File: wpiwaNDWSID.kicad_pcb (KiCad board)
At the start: 2 copper layers, 85.8 x 30 mm, 28 parts, among them J1 USB_C_Receptacle_USB2.0_16P, J2 Conn_01x02, J3 Conn_01x04, J4 Conn_01x06, SW1 SW_Push, SW2 SW_Push, U1 AP63205WU, U2 AP7363-33D-13, U3 ESP32-S3-WROOM-1, U4 74AHCT125

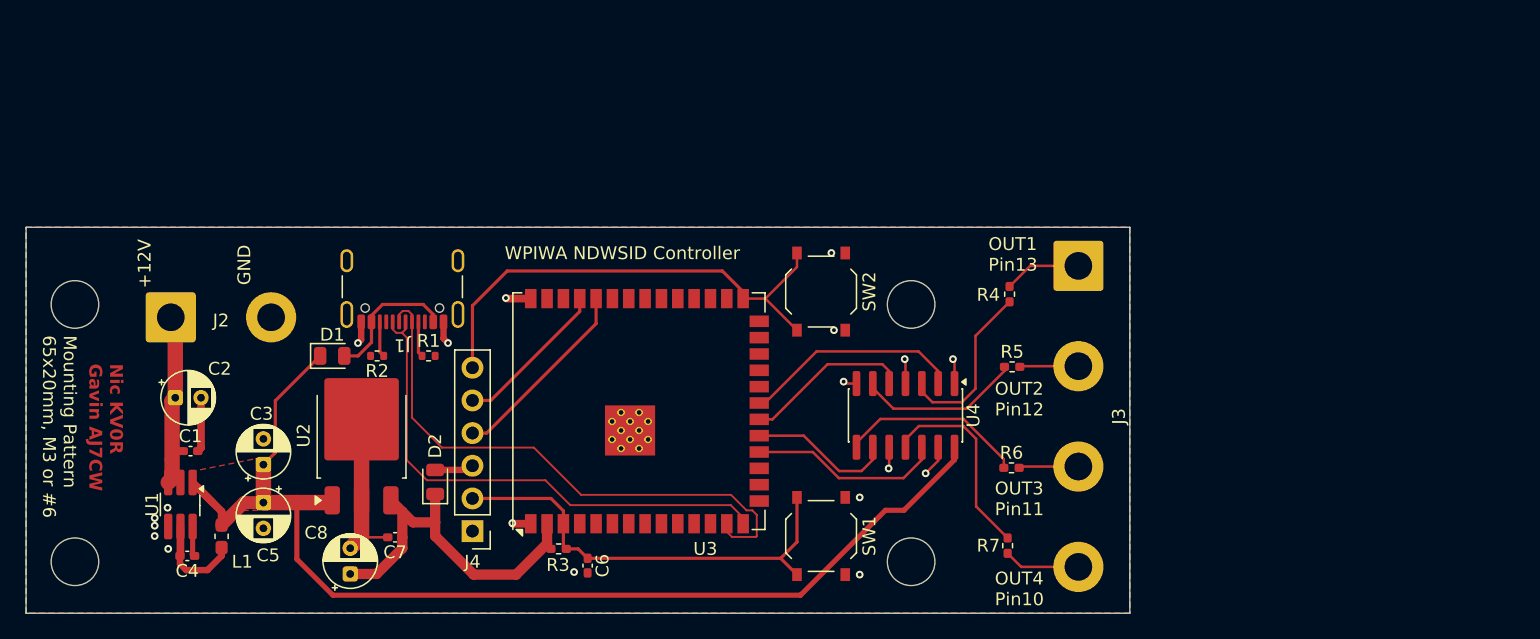
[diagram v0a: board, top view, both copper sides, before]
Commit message: rev 2
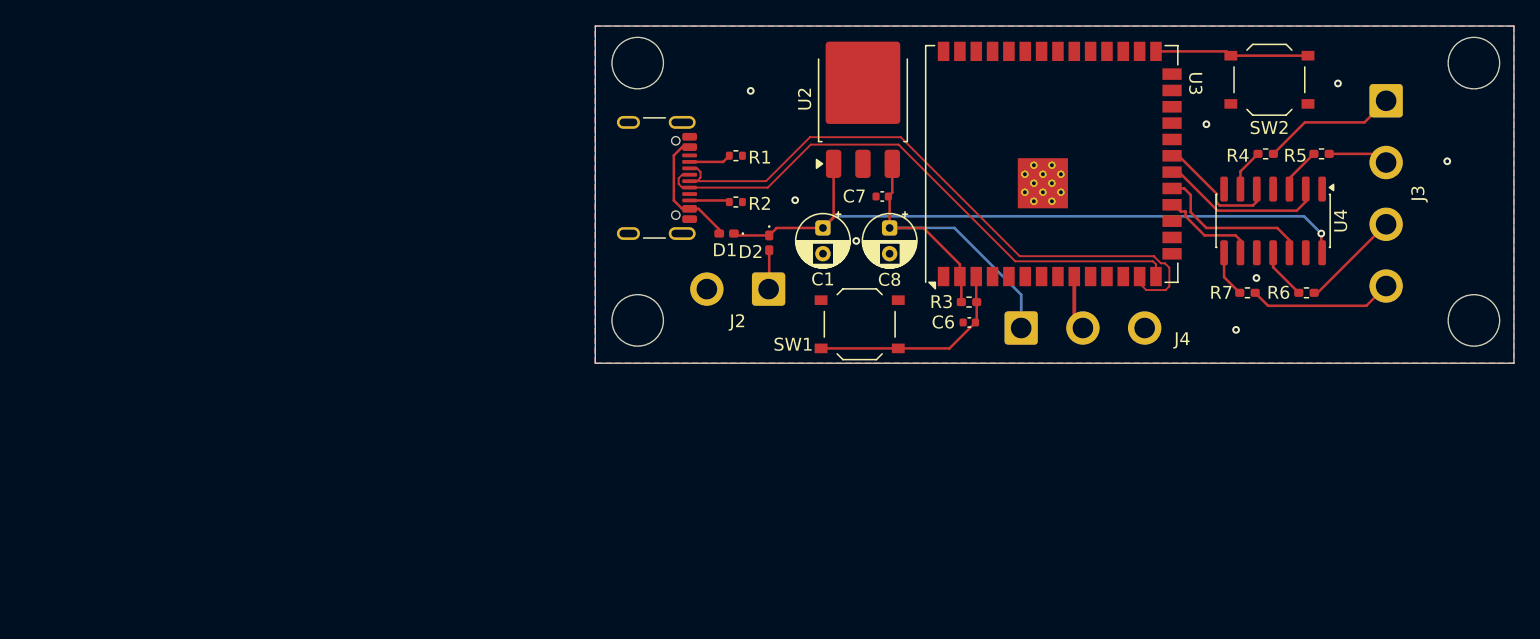
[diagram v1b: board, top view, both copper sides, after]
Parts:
- removed C2: 10uF, Capacitor_THT:CP_Radial_D4.0mm_P2.00mm
- removed C3, C5: 22uF, Capacitor_THT:CP_Radial_D4.0mm_P2.00mm
- removed C4: 0.1uF, Capacitor_SMD:C_0402_1005Metric_Pad0.74x0.62mm_HandSolder
- removed L1: 4.7uH, Inductor_SMD:L_0603_1608Metric_Pad1.05x0.95mm_HandSolder
- removed U1: AP63205WU, Package_TO_SOT_SMD:TSOT-23-6_HandSoldering
- C1: value 0.1uF -> 22uF; footprint Capacitor_SMD:C_0402_1005Metric_Pad0.74x0.62mm_HandSolder -> Capacitor_THT:CP_Radial_D4.0mm_P2.00mm
- C6, C7: footprint Capacitor_SMD:C_0402_1005Metric_Pad0.74x0.62mm_HandSolder -> Capacitor_SMD:C_0402_1005Metric
- D1, D2: footprint Diode_SMD:D_0805_2012Metric -> Diode_SMD:D_0402_1005Metric_Pad0.77x0.64mm_HandSolder
- J2: footprint Connector_Wire:SolderWire-1.5sqmm_1x02_P7.8mm_D1.7mm_OD3.9mm -> Connector_Wire:SolderWire-0.75sqmm_1x02_P4.8mm_D1.25mm_OD2.3mm
- J3: footprint Connector_Wire:SolderWire-1.5sqmm_1x04_P7.8mm_D1.7mm_OD3.9mm -> Connector_Wire:SolderWire-0.75sqmm_1x04_P4.8mm_D1.25mm_OD2.3mm
- J4: value Conn_01x06 -> Conn_01x03; footprint Connector_PinHeader_2.54mm:PinHeader_1x06_P2.54mm_Vertical -> Connector_Wire:SolderWire-0.75sqmm_1x03_P4.8mm_D1.25mm_OD2.3mm
- moved C1 52.1 mm to (180.1, 97.1), turned to -90 degrees
- moved C8 49.8 mm to (185.3, 97.1), turned to -90 degrees
- moved U2 46.9 mm to (183.3, 87.0)
- moved J2 46.5 mm to (175.9, 101.8), turned to 180 degrees
- moved C7 46.2 mm to (184.8, 94.6)
- moved J4 45.5 mm to (195.6, 104.8), turned to 0 degrees
- moved SW2 38.5 mm to (214.8, 85.5), turned to 180 degrees
- moved U3 37.4 mm to (197.9, 92.1)
- moved R3 37.2 mm to (191.5, 102.8)
- moved C6 35.2 mm to (191.5, 104.4), turned to 180 degrees
- moved U4 32.3 mm to (215.1, 96.5)
- moved D1 32.1 mm to (172.7, 97.5), turned to 180 degrees
- moved D2 31.9 mm to (176.0, 98.2), turned to -90 degrees
- moved R2 30.3 mm to (173.4, 95.0), turned to 0 degrees
- moved R5 29.2 mm to (218.9, 91.3)
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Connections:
- C1 pad 1: +12V -> +5V
- C6 pad 1: Net-(J4-Pin_2) -> Net-(U3-EN)
- D2 pad 1: +3.3V -> +5V
- J2 pad 1: +12V -> Net-(D2-A)
- J4 pad 1: GND -> +3.3V
- J4 pad 2: Net-(J4-Pin_2) -> /ESP32/RELAY
- J4 pad 3: Net-(D2-A) -> GND
- R3 pad 2: Net-(J4-Pin_2) -> Net-(U3-EN)
- SW1 pad 2: Net-(J4-Pin_2) -> Net-(U3-EN)
- SW2 pad 2: Net-(J4-Pin_6) -> Net-(U3-IO0)
- U3 pad 26: unconnected-(U3-IO45-Pad26) -> GND
- U3 pad 27: Net-(J4-Pin_6) -> Net-(U3-IO0)
- U3 pad 3: Net-(J4-Pin_2) -> Net-(U3-EN)
- U3 pad 36: Net-(J4-Pin_4) -> unconnected-(U3-RXD0-Pad36)
- U3 pad 37: Net-(J4-Pin_5) -> unconnected-(U3-TXD0-Pad37)
- U3 pad 9: unconnected-(U3-IO16-Pad9) -> /ESP32/RELAY
- U4 pad 11: Net-(R7-Pad1) -> Net-(R6-Pad1)
- U4 pad 12: /ESP32/LED_4 -> /ESP32/LED_3
- U4 pad 2: /ESP32/LED_1 -> /ESP32/LED_2
- U4 pad 3: Net-(R4-Pad1) -> Net-(R5-Pad1)
- U4 pad 5: /ESP32/LED_2 -> /ESP32/LED_1
- U4 pad 6: Net-(R5-Pad1) -> Net-(R4-Pad1)
- U4 pad 8: Net-(R6-Pad1) -> Net-(R7-Pad1)
- U4 pad 9: /ESP32/LED_3 -> /ESP32/LED_4
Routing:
- net Net-(J4-Pin_6): track 37.9 -> 0.00 mm
- net +5V: track 90.6 -> 53.7 mm, vias 0 -> 1
- net Net-(J4-Pin_2): track 35.0 -> 0.00 mm
- net GND: track 34.2 -> 0.00 mm, vias 19 -> 8
- net Net-(U3-EN): track 0.00 -> 16.5 mm
- net Net-(J4-Pin_4): track 15.1 -> 0.00 mm
- net +12V: track 14.6 -> 0.00 mm
- net Net-(J4-Pin_5): track 12.2 -> 0.00 mm
- net Net-(R7-Pad1): track 15.7 -> 3.62 mm
- net Net-(U3-IO0): track 0.00 -> 12.0 mm
- net Net-(R6-Pad1): track 14.5 -> 3.94 mm
- net Net-(R4-Pad1): track 13.4 -> 3.30 mm
- net Net-(R5-Pad1): track 12.8 -> 3.52 mm
- net /ESP32/LED_1: track 17.2 -> 9.68 mm
- net Net-(U1-SW): track 7.46 -> 0.00 mm
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- removed copper zone on F.Cu, net +5V
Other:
- board size 85.8 x 30 mm -> 71.4 x 26.2 mm
- board text removed: "+12V"
- board text removed: "GND"
- board text removed: "Mounting Pattern 65x20mm, M3 or #6"
- board text removed: "Nic KV0R Gavin AJ7CW"
- board text removed: "OUT1 Pin13"
- board text removed: "OUT2 Pin12"
- board text removed: "OUT3 Pin11"
- board text removed: "OUT4 Pin10"
- board text removed: "WPIWA NDWSID Controller"
